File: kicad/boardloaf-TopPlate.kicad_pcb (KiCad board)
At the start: 2 copper layers, 100 x 100 mm, 8 parts

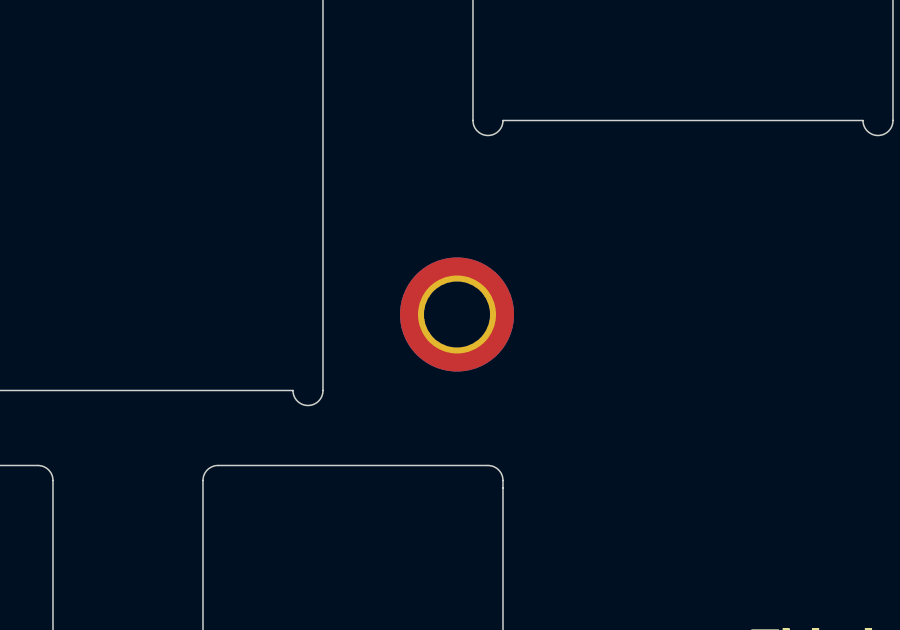
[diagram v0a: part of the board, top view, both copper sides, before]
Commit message: align hole
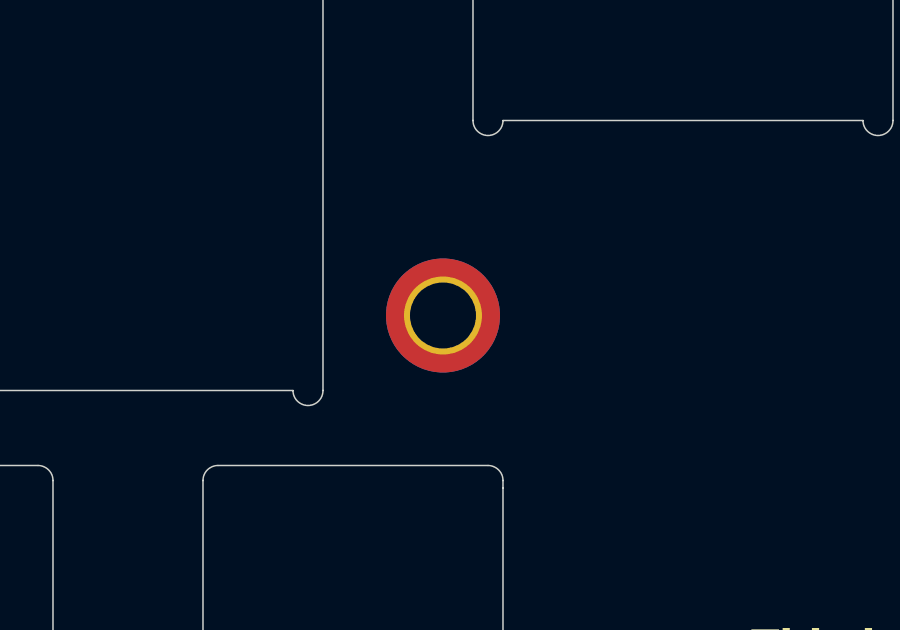
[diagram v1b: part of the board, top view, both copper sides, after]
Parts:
- moved GND 0.47 mm to (85.5, 112.5)
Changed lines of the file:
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@@
 	(footprint "MountingHole:MountingHole_2.2mm_M2_DIN965_Pad_TopBottom"
 		(layer "F.Cu")
-		(at 85.967461 112.466946)
+		(at 85.5 112.5)
 		(descr "Mounting Hole 2.2mm, M2, generated by kicad-footprint-generator mountinghole.py")
 		(tags "mountinghole M2 DIN965")
